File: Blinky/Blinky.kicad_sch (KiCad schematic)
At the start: 12 parts, among them IC1 PAM8303CBSC, J1 TP4056, J2 Battery Connector, J3 Speaker Connector, J4 USB_B_Micro, J5 Charging Notches, SW1 SW_Push, U1 ESP32-S2-WROVER

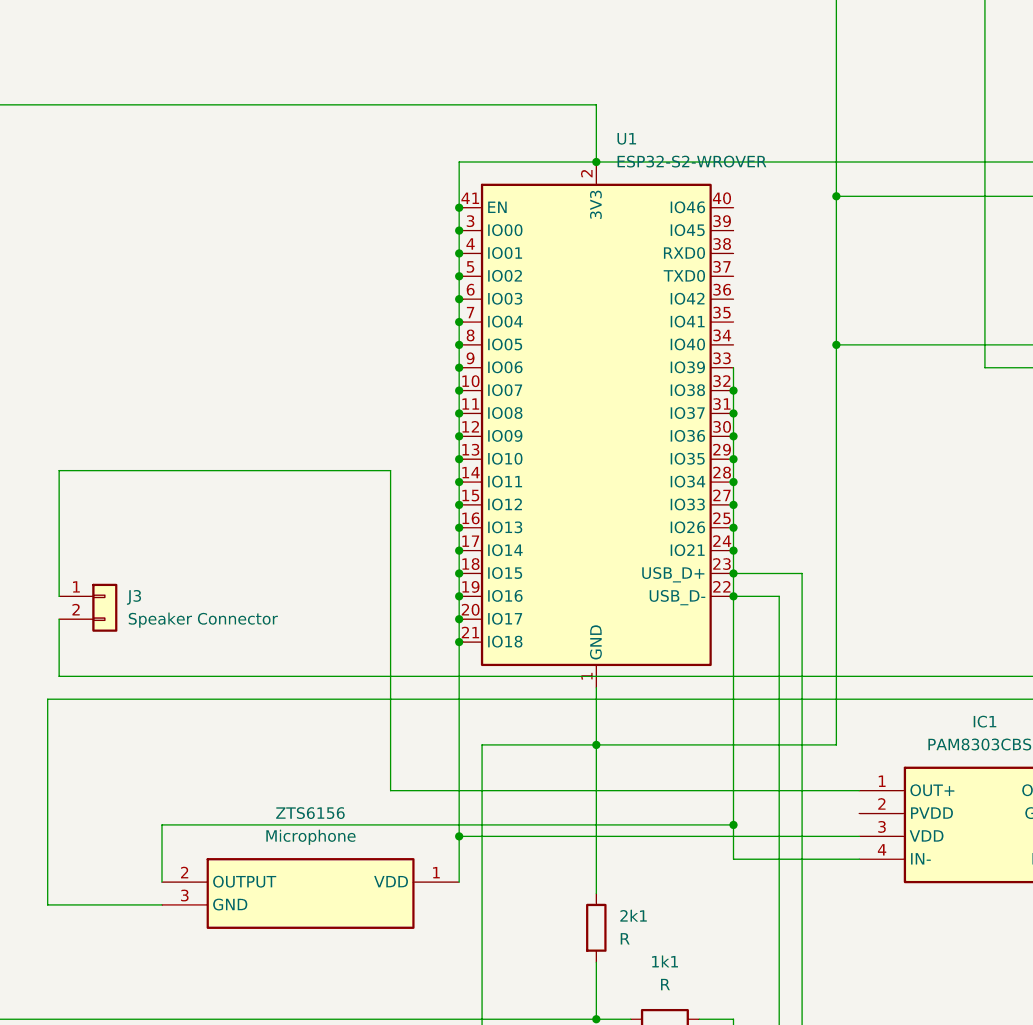
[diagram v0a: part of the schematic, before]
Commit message: bugfix
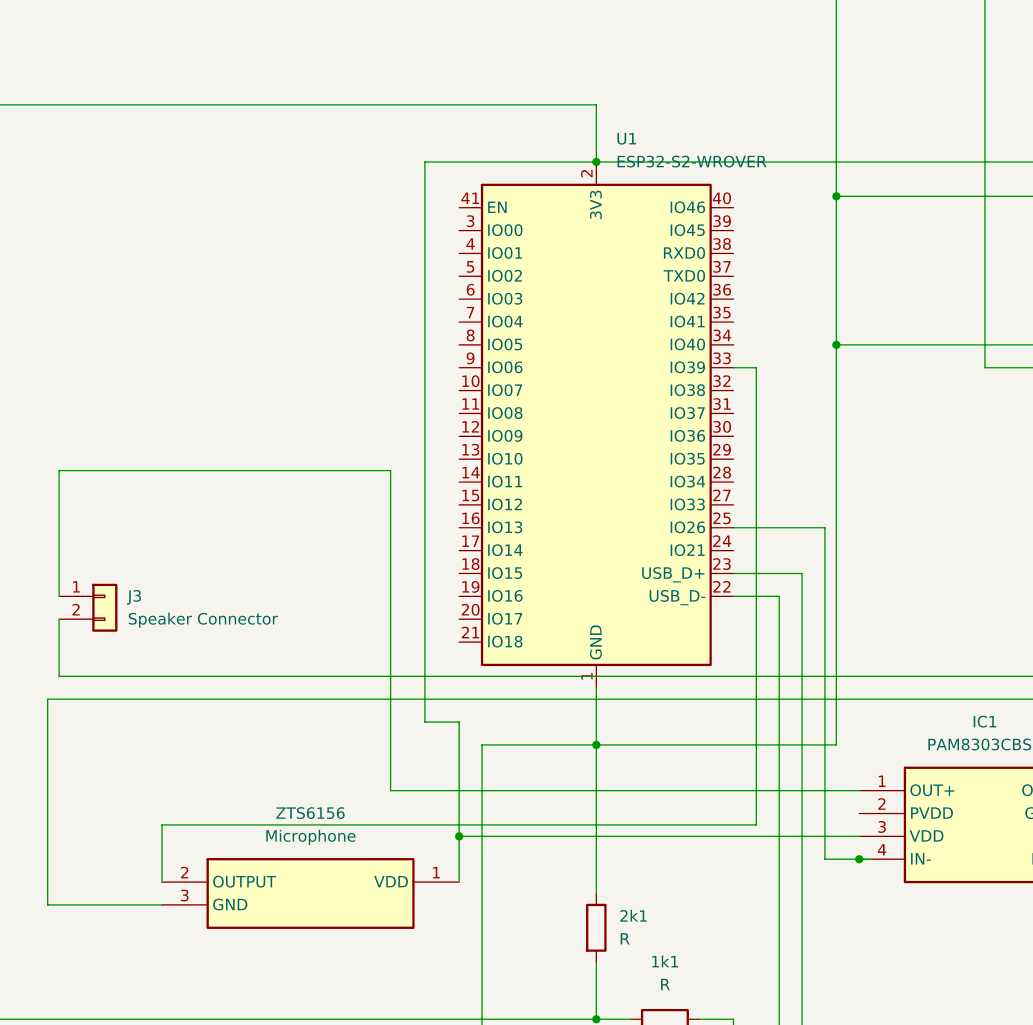
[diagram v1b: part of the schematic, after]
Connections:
- new net: 1k1.1, 2k1.2, IC1.3 (VDD), J1.5 (BAT), J2.1 (Pin_1), SW1.1, U1.2 (3V3), ZTS6156.1 (VDD)
- new net: J4.2 (D-), U1.22 (USB_D-)
- new net: J4.3 (D+), U1.23 (USB_D+)
- new net: U1.33 (IO39), ZTS6156.2 (OUTPUT)
- new net: IC1.4 (IN-), U1.25 (IO26)
- now unconnected: U1.10 (IO07), U1.11 (IO08), U1.12 (IO09), U1.13 (IO10), U1.14 (IO11), U1.15 (IO12), U1.16 (IO13), U1.17 (IO14), U1.18 (IO15), U1.19 (IO16), U1.20 (IO17), U1.21 (IO18), U1.24 (IO21), U1.27 (IO33), U1.28 (IO34), U1.29 (IO35), U1.3 (IO00), U1.30 (IO36), U1.31 (IO37), U1.32 (IO38), U1.4 (IO01), U1.41 (EN), U1.5 (IO02), U1.6 (IO03), U1.7 (IO04), U1.8 (IO05), U1.9 (IO06)
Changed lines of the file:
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@@
 (kicad_sch (version 20230121) (generator eeschema)
   (paper "A4")
-  (junction (at 130.81 96.52) (diameter 0) (color 0 0 0 0)
-  )
-  (junction (at 130.81 101.6) (diameter 0) (color 0 0 0 0)
-  )
   (junction (at 146.05 48.26) (diameter 0) (color 0 0 0 0)
   )
-  (junction (at 130.81 88.9) (diameter 0) (color 0 0 0 0)
-  )
   (junction (at 237.49 48.26) (diameter 0) (color 0 0 0 0)
   )
-  (junction (at 130.81 71.12) (diameter 0) (color 0 0 0 0)
-  )
-  (junction (at 130.81 86.36) (diameter 0) (color 0 0 0 0)
-  )
-  (junction (at 161.29 76.2) (diameter 0) (color 0 0 0 0)
-  )
-  (junction (at 130.81 93.98) (diameter 0) (color 0 0 0 0)
-  )
-  (junction (at 161.29 121.92) (diameter 0) (color 0 0 0 0)
-  )
-  (junction (at 130.81 53.34) (diameter 0) (color 0 0 0 0)
-  )
   (junction (at 146.05 143.51) (diameter 0) (color 0 0 0 0)
   )
-  (junction (at 130.81 68.58) (diameter 0) (color 0 0 0 0)
-  )
-  (junction (at 130.81 99.06) (diameter 0) (color 0 0 0 0)
-  )
-  (junction (at 130.81 81.28) (diameter 0) (color 0 0 0 0)
+  (junction (at 175.26 125.73) (diameter 0) (color 0 0 0 0)
   )
   (junction (at 146.05 113.03) (diameter 0) (color 0 0 0 0)
   )
-  (junction (at 161.29 88.9) (diameter 0) (color 0 0 0 0)
-  )
-  (junction (at 130.81 76.2) (diameter 0) (color 0 0 0 0)
-  )
-  (junction (at 130.81 91.44) (diameter 0) (color 0 0 0 0)
-  )
-  (junction (at 161.29 81.28) (diameter 0) (color 0 0 0 0)
-  )
-  (junction (at 161.29 83.82) (diameter 0) (color 0 0 0 0)
-  )
-  (junction (at 161.29 86.36) (diameter 0) (color 0 0 0 0)
-  )
-  (junction (at 130.81 55.88) (diameter 0) (color 0 0 0 0)
-  )
   (junction (at 172.72 52.07) (diameter 0) (color 0 0 0 0)
   )
-  (junction (at 161.29 96.52) (diameter 0) (color 0 0 0 0)
-  )
-  (junction (at 130.81 58.42) (diameter 0) (color 0 0 0 0)
-  )
-  (junction (at 161.29 91.44) (diameter 0) (color 0 0 0 0)
-  )
   (junction (at 130.81 123.19) (diameter 0) (color 0 0 0 0)
   )
-  (junction (at 130.81 63.5) (diameter 0) (color 0 0 0 0)
-  )
   (junction (at 254 73.66) (diameter 0) (color 0 0 0 0)
   )
-  (junction (at 130.81 83.82) (diameter 0) (color 0 0 0 0)
-  )
-  (junction (at 130.81 78.74) (diameter 0) (color 0 0 0 0)
-  )
-  (junction (at 161.29 93.98) (diameter 0) (color 0 0 0 0)
-  )
-  (junction (at 130.81 73.66) (diameter 0) (color 0 0 0 0)
-  )
-  (junction (at 161.29 73.66) (diameter 0) (color 0 0 0 0)
-  )
   (junction (at 237.49 49.53) (diameter 0) (color 0 0 0 0)
   )
-  (junction (at 130.81 60.96) (diameter 0) (color 0 0 0 0)
-  )
-  (junction (at 161.29 78.74) (diameter 0) (color 0 0 0 0)
-  )
   (junction (at 172.72 68.58) (diameter 0) (color 0 0 0 0)
   )
-  (junction (at 130.81 66.04) (diameter 0) (color 0 0 0 0)
-  )
   (wire (pts (xy 146.05 143.51) (xy 146.05 137.16))
     (stroke (width 0) (type default))
@@
     (stroke (width 0) (type default))
   )
-  (wire (pts (xy 130.81 55.88) (xy 130.81 58.42))
-    (stroke (width 0) (type default))
-  )
   (wire (pts (xy 254 39.37) (xy 237.49 39.37))
     (stroke (width 0) (type default))
   )
-  (wire (pts (xy 130.81 101.6) (xy 130.81 123.19))
-    (stroke (width 0) (type default))
-  )
-  (wire (pts (xy 130.81 96.52) (xy 130.81 99.06))
+  (wire (pts (xy 127 110.49) (xy 130.81 110.49))
     (stroke (width 0) (type default))
   )
@@
     (stroke (width 0) (type default))
   )
+  (wire (pts (xy 130.81 110.49) (xy 130.81 123.19))
+    (stroke (width 0) (type default))
+  )
+  (wire (pts (xy 171.45 88.9) (xy 171.45 125.73))
+    (stroke (width 0) (type default))
+  )
   (wire (pts (xy 237.49 48.26) (xy 237.49 49.53))
     (stroke (width 0) (type default))
@@
     (stroke (width 0) (type default))
   )
-  (wire (pts (xy 130.81 71.12) (xy 130.81 73.66))
-    (stroke (width 0) (type default))
-  )
   (wire (pts (xy 130.81 123.19) (xy 130.81 128.27))
     (stroke (width 0) (type default))
   )
-  (wire (pts (xy 130.81 86.36) (xy 130.81 88.9))
-    (stroke (width 0) (type default))
-  )
   (wire (pts (xy 237.49 52.07) (xy 172.72 52.07))
     (stroke (width 0) (type default))
@@
     (stroke (width 0) (type default))
   )
+  (wire (pts (xy 127 48.26) (xy 127 110.49))
+    (stroke (width 0) (type default))
+  )
   (wire (pts (xy 238.76 52.07) (xy 238.76 90.17))
     (stroke (width 0) (type default))
@@
     (stroke (width 0) (type default))
   )
+  (wire (pts (xy 163.83 121.92) (xy 97.79 121.92))
+    (stroke (width 0) (type default))
+  )
   (wire (pts (xy 161.29 143.51) (xy 157.48 143.51))
     (stroke (width 0) (type default))
   )
-  (wire (pts (xy 130.81 66.04) (xy 130.81 68.58))
-    (stroke (width 0) (type default))
-  )
   (wire (pts (xy 140.97 173.99) (xy 140.97 168.91))
     (stroke (width 0) (type default))
   )
-  (wire (pts (xy 130.81 91.44) (xy 130.81 93.98))
-    (stroke (width 0) (type default))
-  )
   (wire (pts (xy 97.79 121.92) (xy 97.79 128.27))
     (stroke (width 0) (type default))
@@
     (stroke (width 0) (type default))
   )
-  (wire (pts (xy 130.81 83.82) (xy 130.81 86.36))
-    (stroke (width 0) (type default))
-  )
-  (wire (pts (xy 130.81 53.34) (xy 130.81 55.88))
+  (wire (pts (xy 175.26 125.73) (xy 176.53 125.73))
     (stroke (width 0) (type default))
   )
@@
     (stroke (width 0) (type default))
   )
-  (wire (pts (xy 161.29 78.74) (xy 161.29 81.28))
-    (stroke (width 0) (type default))
-  )
-  (wire (pts (xy 130.81 93.98) (xy 130.81 96.52))
-    (stroke (width 0) (type default))
-  )
   (wire (pts (xy 77.47 143.51) (xy 146.05 143.51))
     (stroke (width 0) (type default))
   )
-  (wire (pts (xy 130.81 81.28) (xy 130.81 83.82))
+  (wire (pts (xy 161.29 71.12) (xy 163.83 71.12))
     (stroke (width 0) (type default))
   )
@@
     (stroke (width 0) (type default))
   )
-  (wire (pts (xy 161.29 91.44) (xy 161.29 93.98))
-    (stroke (width 0) (type default))
-  )
-  (wire (pts (xy 161.29 76.2) (xy 161.29 78.74))
-    (stroke (width 0) (type default))
-  )
   (wire (pts (xy 77.47 143.51) (xy 77.47 41.91))
     (stroke (width 0) (type default))
   )
-  (wire (pts (xy 130.81 60.96) (xy 130.81 63.5))
-    (stroke (width 0) (type default))
-  )
   (wire (pts (xy 172.72 68.58) (xy 172.72 113.03))
     (stroke (width 0) (type default))
   )
-  (wire (pts (xy 161.29 93.98) (xy 161.29 96.52))
-    (stroke (width 0) (type default))
-  )
-  (wire (pts (xy 130.81 68.58) (xy 130.81 71.12))
-    (stroke (width 0) (type default))
-  )
-  (wire (pts (xy 146.05 48.26) (xy 130.81 48.26))
-    (stroke (width 0) (type default))
-  )
-  (wire (pts (xy 130.81 73.66) (xy 130.81 76.2))
-    (stroke (width 0) (type default))
-  )
-  (wire (pts (xy 161.29 121.92) (xy 97.79 121.92))
-    (stroke (width 0) (type default))
-  )
-  (wire (pts (xy 161.29 88.9) (xy 161.29 91.44))
-    (stroke (width 0) (type default))
-  )
-  (wire (pts (xy 130.81 63.5) (xy 130.81 66.04))
-    (stroke (width 0) (type default))
-  )
-  (wire (pts (xy 161.29 71.12) (xy 161.29 73.66))
+  (wire (pts (xy 127 48.26) (xy 146.05 48.26))
     (stroke (width 0) (type default))
   )
@@
     (stroke (width 0) (type default))
   )
-  (wire (pts (xy 161.29 86.36) (xy 161.29 88.9))
-    (stroke (width 0) (type default))
-  )
   (wire (pts (xy 148.59 158.75) (xy 168.91 158.75))
     (stroke (width 0) (type default))
   )
-  (wire (pts (xy 130.81 76.2) (xy 130.81 78.74))
-    (stroke (width 0) (type default))
-  )
-  (wire (pts (xy 130.81 58.42) (xy 130.81 60.96))
-    (stroke (width 0) (type default))
-  )
   (wire (pts (xy 237.49 49.53) (xy 236.22 49.53))
     (stroke (width 0) (type default))
@@
     (stroke (width 0) (type default))
   )
-  (wire (pts (xy 161.29 73.66) (xy 161.29 76.2))
-    (stroke (width 0) (type default))
-  )
-  (wire (pts (xy 130.81 48.26) (xy 130.81 53.34))
+  (wire (pts (xy 163.83 71.12) (xy 163.83 121.92))
     (stroke (width 0) (type default))
   )
@@
     (stroke (width 0) (type default))
   )
-  (wire (pts (xy 161.29 121.92) (xy 161.29 125.73))
-    (stroke (width 0) (type default))
-  )
   (wire (pts (xy 123.19 82.55) (xy 123.19 118.11))
     (stroke (width 0) (type default))
@@
     (stroke (width 0) (type default))
   )
-  (wire (pts (xy 130.81 88.9) (xy 130.81 91.44))
-    (stroke (width 0) (type default))
-  )
-  (wire (pts (xy 161.29 96.52) (xy 161.29 121.92))
-    (stroke (width 0) (type default))
-  )
   (wire (pts (xy 203.2 120.65) (xy 210.82 120.65))
     (stroke (width 0) (type default))
@@
     (stroke (width 0) (type default))
   )
-  (wire (pts (xy 161.29 83.82) (xy 161.29 86.36))
-    (stroke (width 0) (type default))
-  )
   (wire (pts (xy 189.23 26.67) (xy 189.23 71.12))
     (stroke (width 0) (type default))
   )
-  (wire (pts (xy 130.81 99.06) (xy 130.81 101.6))
+  (wire (pts (xy 161.29 88.9) (xy 171.45 88.9))
     (stroke (width 0) (type default))
   )
@@
     (stroke (width 0) (type default))
   )
-  (wire (pts (xy 130.81 78.74) (xy 130.81 81.28))
-    (stroke (width 0) (type default))
-  )
-  (wire (pts (xy 161.29 81.28) (xy 161.29 83.82))
-    (stroke (width 0) (type default))
-  )
-  (wire (pts (xy 161.29 125.73) (xy 175.26 125.73))
+  (wire (pts (xy 171.45 125.73) (xy 175.26 125.73))
     (stroke (width 0) (type default))
   )
@@
     )
     (pin "1")
+    (pin "2")
     (pin "3")
-    (pin "2")
-    (instances
-      (project "Blinky"
+    (instances
+      (project "Blinky"

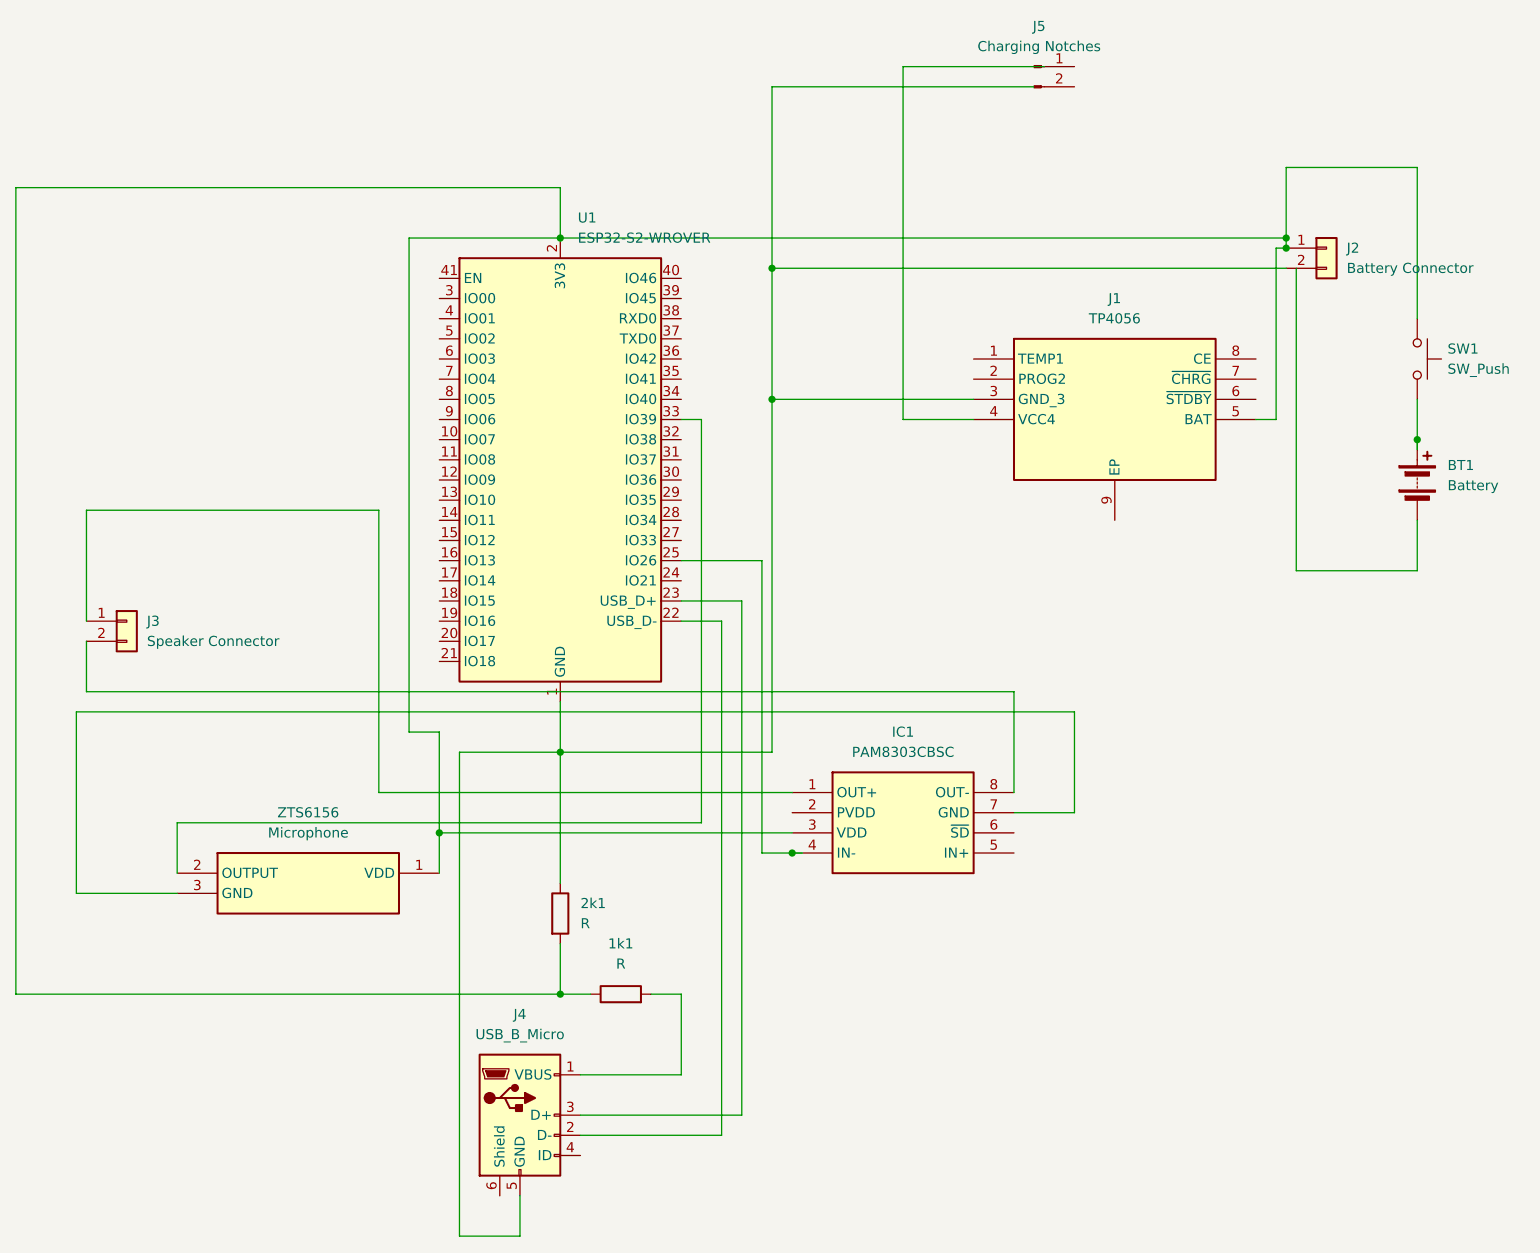
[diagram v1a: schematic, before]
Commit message: bugfix
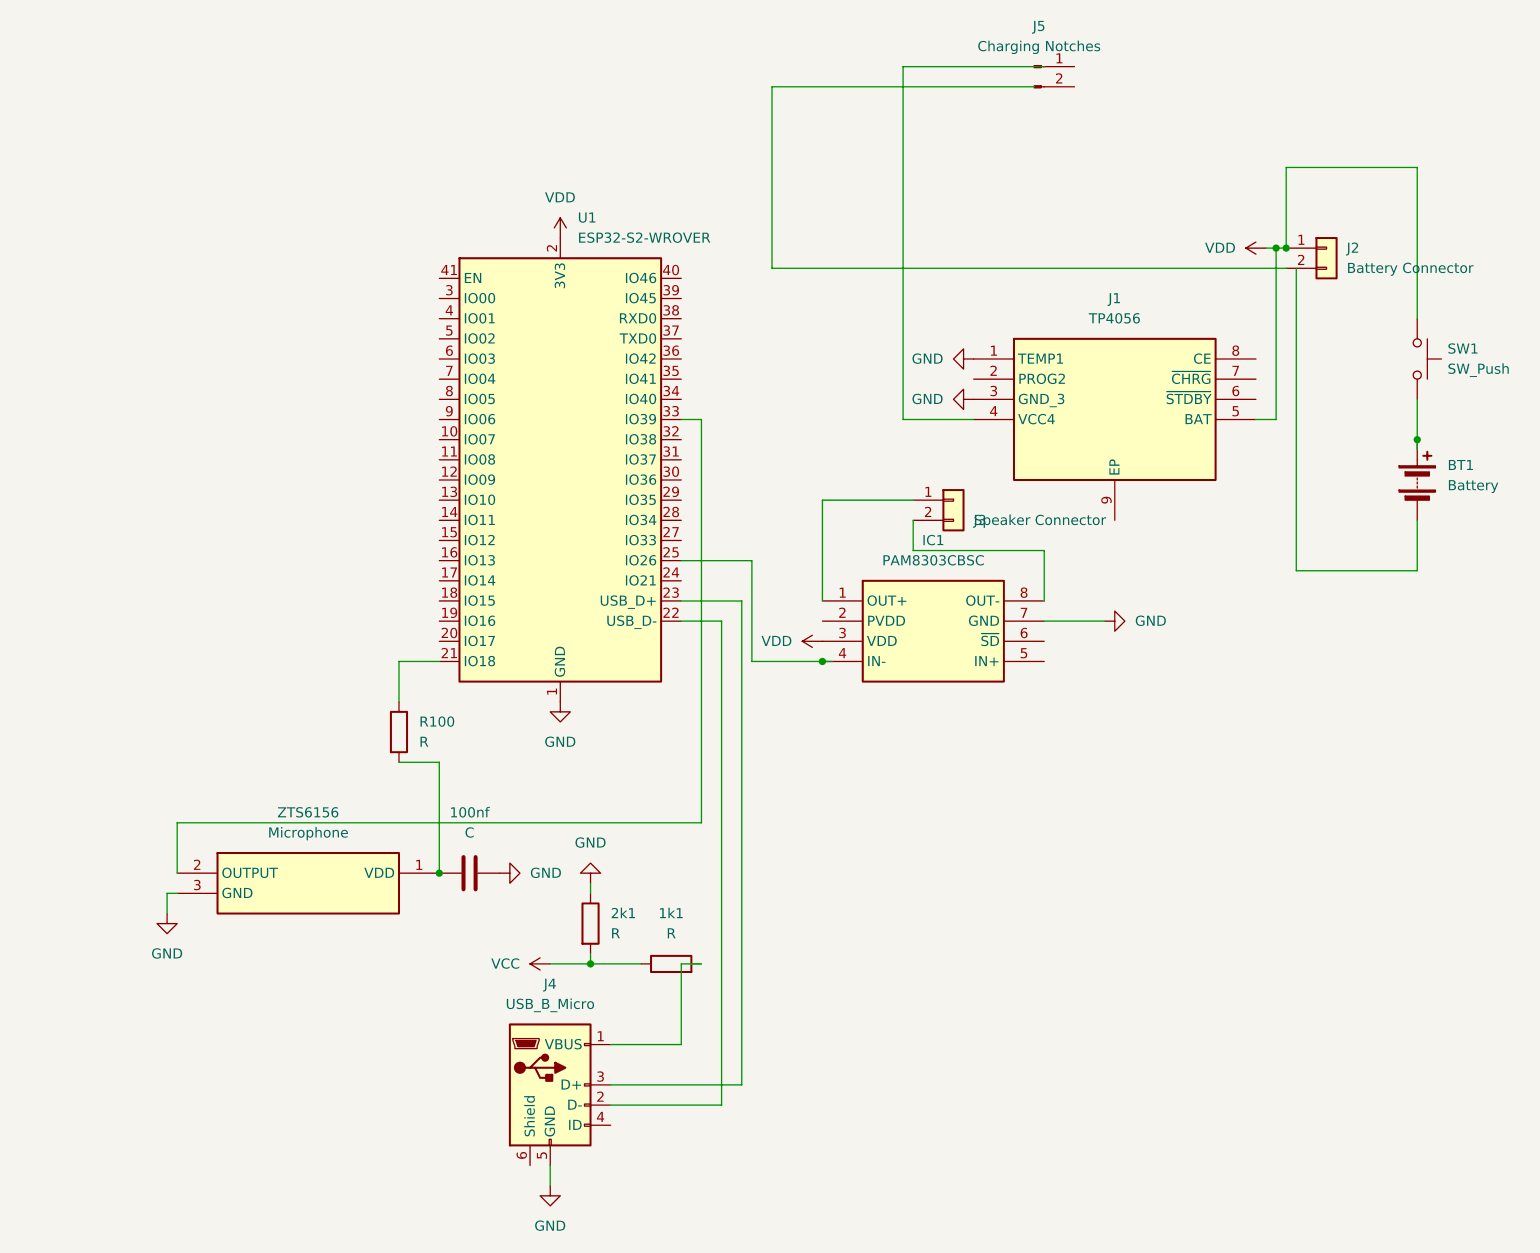
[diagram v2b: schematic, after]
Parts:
- added 100nf: C, symbol Device:C
- added R100: R, symbol Device:R
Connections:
- net VDD: now reaches IC1.3 (VDD), J1.5 (BAT), J2.1 (Pin_1), SW1.1, U1.2 (3V3)
- net VDD: no longer 1k1.1, 2k1.2, ZTS6156.1 (VDD)
- net GND: now reaches J1.1 (TEMP1)
- net GND: now also 2k1.1, IC1.7 (GND), J1.3 (GND_3), J4.5 (GND), U1.1 (GND), U1.26 (GND), U1.42 (GND), U1.43 (GND), ZTS6156.3 (GND), 100nf.2
- net at U1.21 (IO18): now also R100.1
- new net: 100nf.1, R100.2, ZTS6156.1 (VDD)
- new net VCC: 1k1.1, 2k1.2
- now unconnected: J2.2 (Pin_2)
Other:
- moved on the sheet: 1k1, 2k1, IC1, J3, J4
